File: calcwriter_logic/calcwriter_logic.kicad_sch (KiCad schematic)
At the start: 42 parts, among them CON1 FH12-40S-0.5SH_55_, IC1 MAX335CWG_T, IC2 MAX335CWG_T, IC3 MAX335CWG_T, IC4 MAX335CWG_T, J1 USB_C_Receptacle_USB2.0_14P, U1 ATmega32U4-A, U2 ME6211C15M5G-N, Y1 16MHz

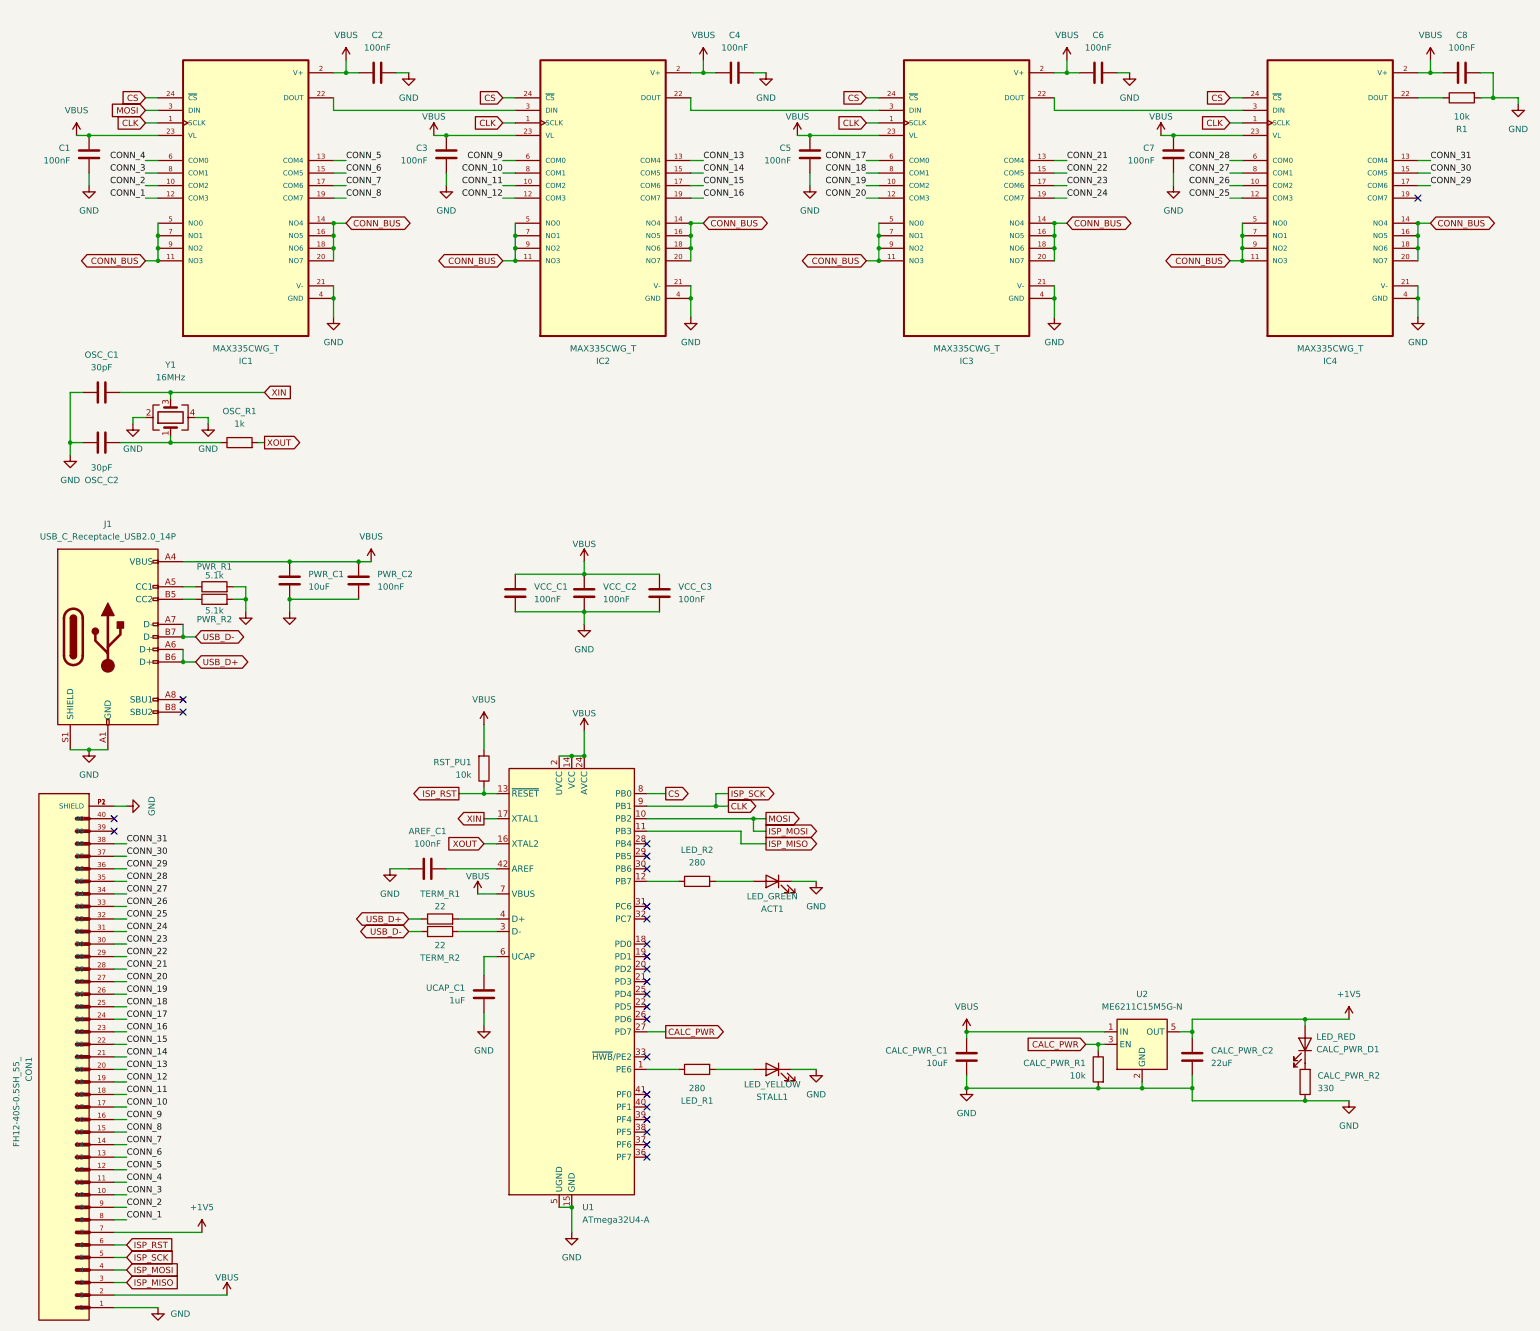
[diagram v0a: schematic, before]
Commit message: did another thing AAAAAAAAAAAAAAAAAAA
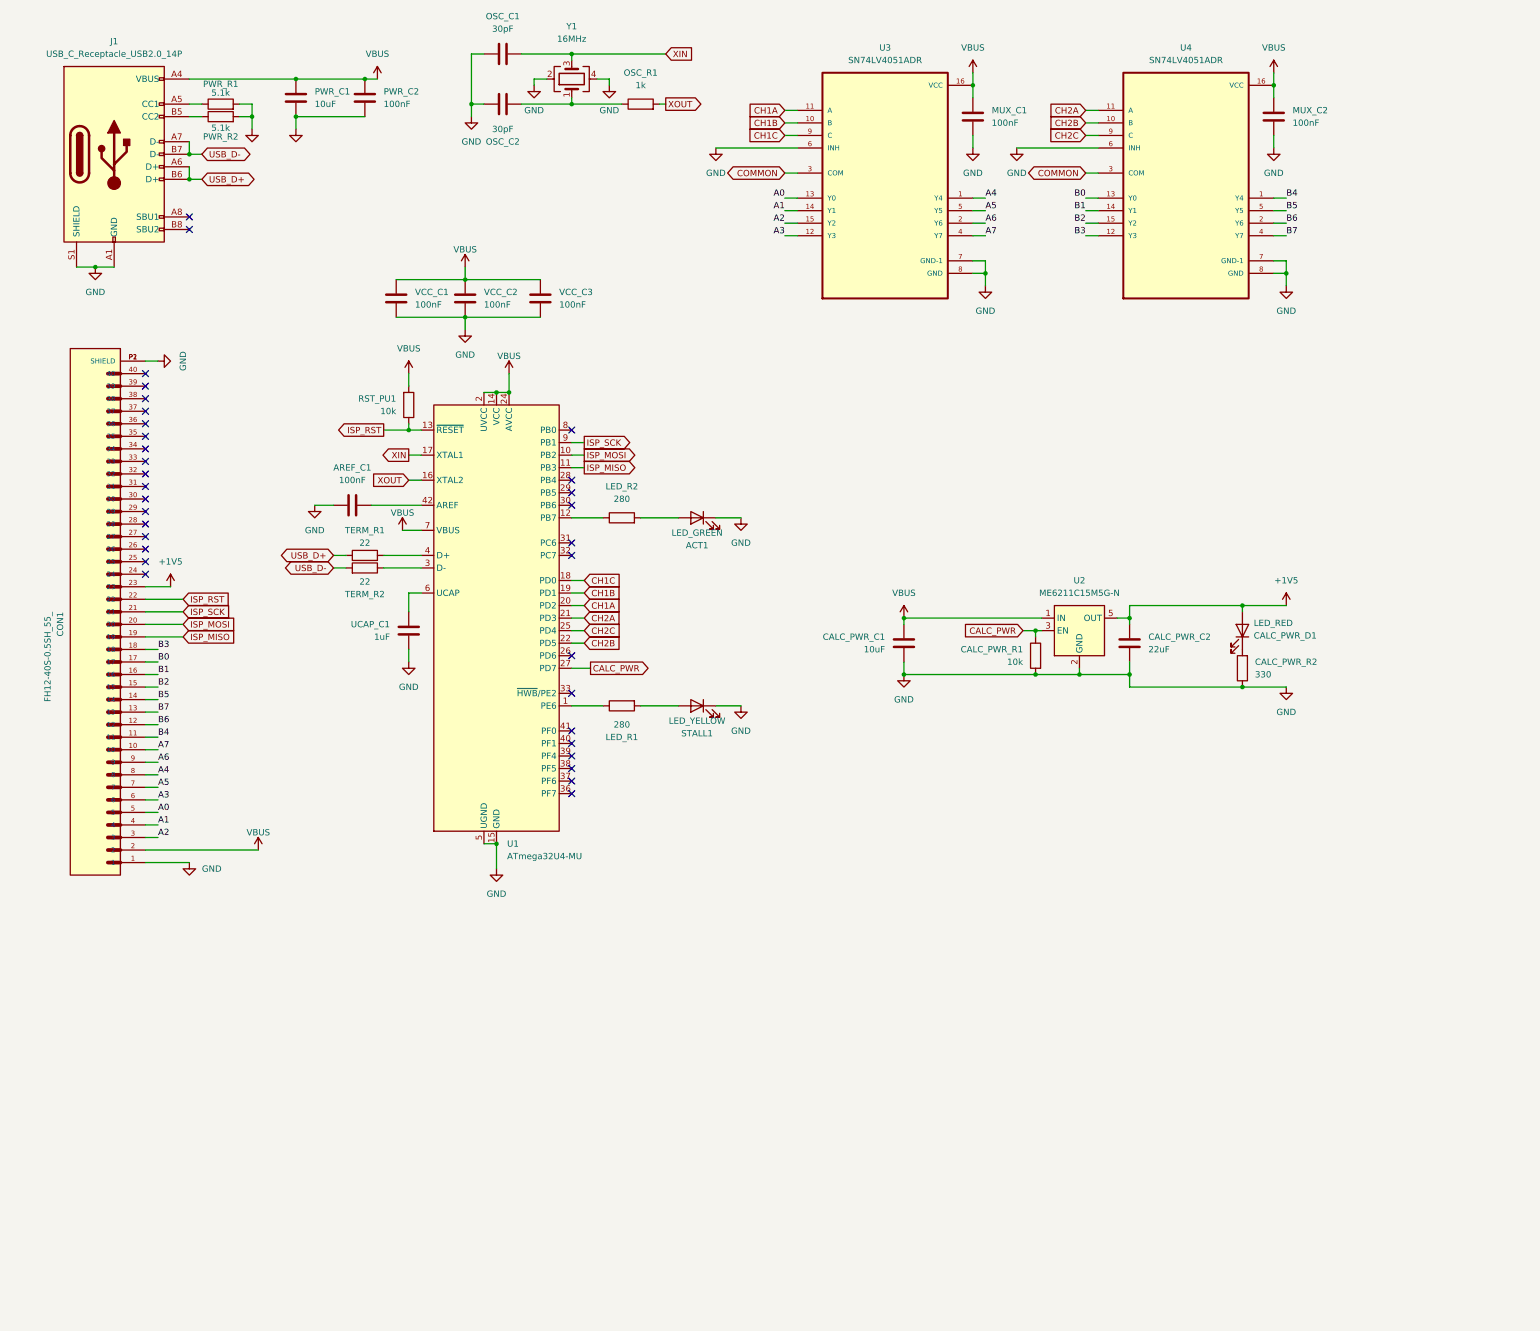
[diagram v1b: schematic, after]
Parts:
- removed C1, C2, C3, C4, C5, C6, C7, C8: 100nF, Capacitor_SMD:C_0402_1005Metric, symbol Device:C
- removed IC1, IC2, IC3, IC4: MAX335CWG_T, MAX335CWG_T:SOIC127P1032X265-24N, symbol MAX335CWG_T:MAX335CWG_T
- removed R1: 10k, Resistor_SMD:R_0402_1005Metric, symbol Device:R
- added MUX_C1, MUX_C2: 100nF, Capacitor_SMD:C_0402_1005Metric, symbol Device:C
- added U3, U4: SN74LV4051ADR, SN74LV4051ADR:SOIC127P600X175-16N, symbol SN74LV4051ADR:SN74LV4051ADR
- U1: value ATmega32U4-A -> ATmega32U4-MU
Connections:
- net CONN_12 is gone; now on net ISP_MISO: CON1.19
- net CONN_13 is gone; now on net ISP_MOSI: CON1.20
- net CONN_15 is gone; now on net ISP_RST: CON1.22
- net CONN_16 is gone; now on net +1V5: CON1.23
- net +1V5: no longer CON1.7
- net GND: now also MUX_C1.1, MUX_C2.1, U3.6 (INH), U3.7 (GND-1), U3.8 (GND), U4.6 (INH), U4.7 (GND-1), U4.8 (GND)
- net ISP_MISO: no longer CON1.3
- net ISP_MOSI: no longer CON1.4
- net ISP_RST: no longer CON1.6
- net VBUS: now also MUX_C1.2, MUX_C2.2, U3.16 (VCC), U4.16 (VCC)
- net CH1C: now reaches U1.18 (PD0)
- net CH1C: now also U3.9 (C)
- net CH1B: now reaches U1.19 (PD1)
- net CH1B: now also U3.10 (B)
- net CH1A: now reaches U1.20 (PD2)
- net CH1A: now also U3.11 (A)
- net CH2A: now reaches U1.21 (PD3)
- net CH2A: now also U4.11 (A)
- net CH2B: now reaches U1.22 (PD5)
- net CH2B: now also U4.10 (B)
- net CH2C: now reaches U1.25 (PD4)
- net CH2C: now also U4.9 (C)
- net CLK renamed A0
- net A0: now also U3.13 (Y0); no longer U1.9 (PB1)
- net CONN_1 renamed A4
- net A4: now also U3.1 (Y4)
- net CONN_10 renamed B0
- net B0: now also U4.13 (Y0)
- net CONN_11 renamed B3
- net B3: now also U4.12 (Y3)
- net CONN_14 renamed ISP_SCK
- net ISP_SCK: now also U1.9 (PB1)
- net CONN_17: no longer names the net of CON1.24
- net CONN_18: no longer names the net of CON1.25
- net CONN_19: no longer names the net of CON1.26
- net CONN_2 renamed A6
- net A6: now also U3.2 (Y6)
- net CONN_20: no longer names the net of CON1.27
- net CONN_21: no longer names the net of CON1.28
- net CONN_22: no longer names the net of CON1.29
- net CONN_23: no longer names the net of CON1.30
- net CONN_24: no longer names the net of CON1.31
- net CONN_25: no longer names the net of CON1.32
- net CONN_26: no longer names the net of CON1.33
- net CONN_27: no longer names the net of CON1.34
- net CONN_28: no longer names the net of CON1.35
- net CONN_29: no longer names the net of CON1.36
- net CONN_3 renamed A7
- net A7: now also U3.4 (Y7)
- net CONN_30: no longer names the net of CON1.37
- net CONN_31: no longer names the net of CON1.38
- net CONN_4 renamed B4
- net B4: now also U4.1 (Y4)
- net CONN_5 renamed B6
- net B6: now also U4.2 (Y6)
- net CONN_6 renamed B7
- net B7: now also U4.4 (Y7)
- net CONN_7 renamed B5
- net B5: now also U4.5 (Y5)
- net CONN_8 renamed B2
- net B2: now also U4.15 (Y2)
- net CONN_9 renamed B1
- net B1: now also U4.14 (Y1)
- net CS: no longer names the net of U1.8 (PB0)
- new net A1: CON1.4, U3.14 (Y1)
- new net A2: CON1.3, U3.15 (Y2)
- new net A3: CON1.6, U3.12 (Y3)
- new net A5: CON1.7, U3.5 (Y5)
- new net COMMON: U3.3 (COM), U4.3 (COM)
- no-connect marks 24 -> 33
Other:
- moved on the sheet: ACT1, AREF_C1, CALC_PWR_C1, CALC_PWR_C2, CALC_PWR_D1, CALC_PWR_R1, CALC_PWR_R2, CON1, J1, LED_R1, LED_R2, OSC_C1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
